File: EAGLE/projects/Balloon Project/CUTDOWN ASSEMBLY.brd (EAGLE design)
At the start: 100 x 100 mm, 2 parts

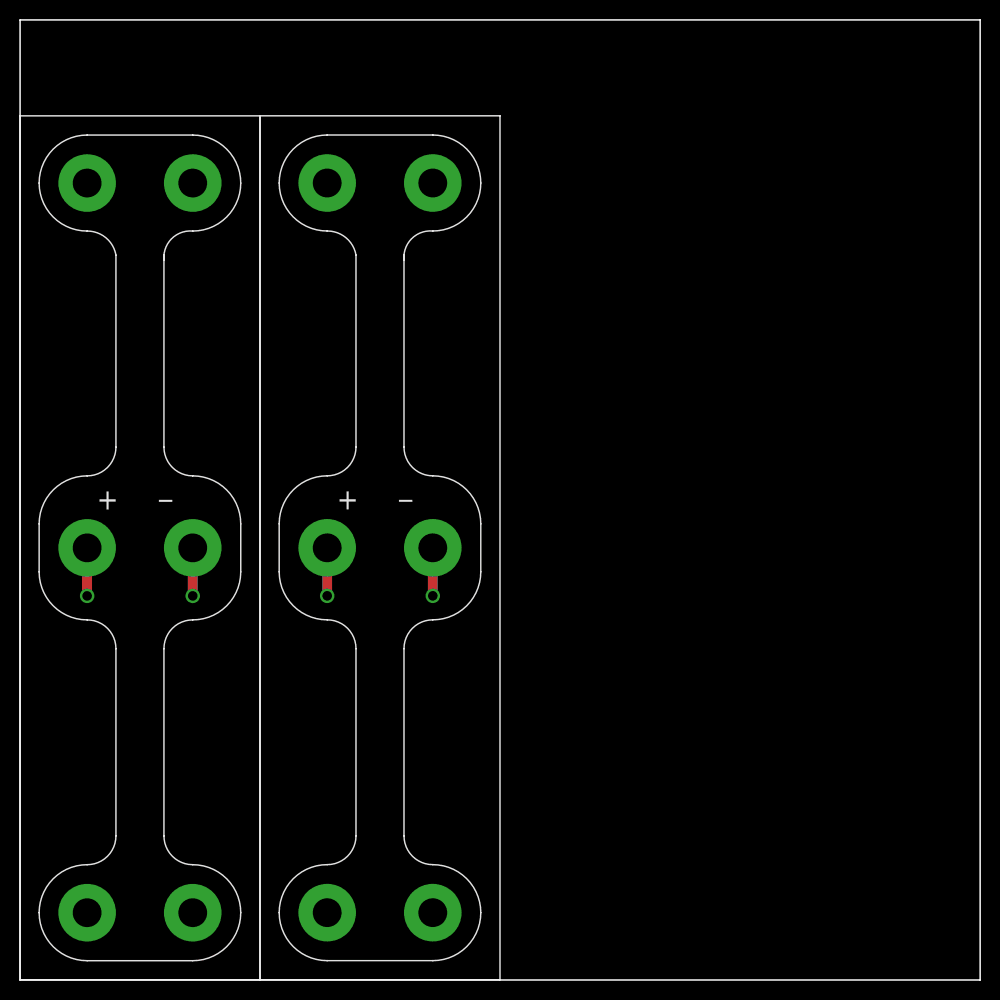
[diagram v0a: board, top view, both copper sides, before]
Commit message: gerber files generated
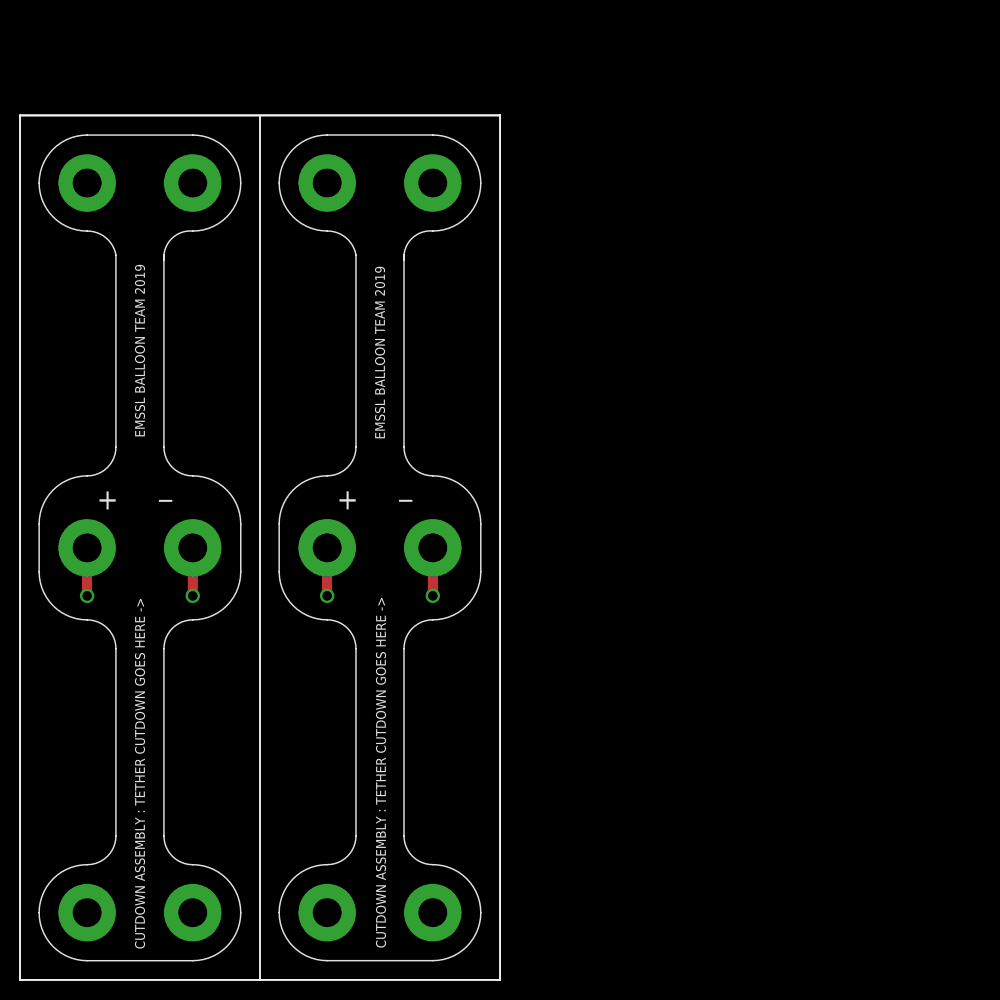
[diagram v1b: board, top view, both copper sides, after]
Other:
- board size 100 x 100 mm -> 50 x 90.1 mm
- board text added: "+"
- board text added: "CUTDOWN ASSEMBLY : TETHER CUTDOWN GOES HERE ->"
- board text added: "EMSSL BALLOON TEAM 2019"
- board text added: "_"
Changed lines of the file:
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@@
 <board>
 <plain>
-<wire x1="0" y1="0" x2="0" y2="100" width="0.1524" layer="20"/>
-<wire x1="0" y1="100" x2="100" y2="100" width="0.1524" layer="20"/>
-<wire x1="100" y1="100" x2="100" y2="0" width="0.1524" layer="20"/>
-<wire x1="100" y1="0" x2="0" y2="0" width="0.1524" layer="20"/>
+<wire x1="0" y1="0" x2="0" y2="90.1" width="0.1524" layer="20"/>
+<wire x1="0" y1="90.1" x2="50" y2="90.1" width="0.1524" layer="20"/>
+<wire x1="50" y1="90.1" x2="50" y2="0" width="0.1524" layer="20"/>
+<wire x1="50" y1="0" x2="0" y2="0" width="0.1524" layer="20"/>
+<text x="13" y="56.5" size="1.016" layer="21" rot="R90">EMSSL BALLOON TEAM 2019</text>
+<text x="38" y="56.3" size="1.016" layer="21" rot="R90">EMSSL BALLOON TEAM 2019</text>
+<text x="38.1" y="3.3" size="1.016" layer="21" rot="R90">CUTDOWN ASSEMBLY : TETHER CUTDOWN GOES HERE -&gt;</text>
+<text x="13" y="3.2" size="1.016" layer="21" rot="R90">CUTDOWN ASSEMBLY : TETHER CUTDOWN GOES HERE -&gt;</text>
+<text x="37.1" y="3.3" size="1.016" layer="22" rot="MR90">CUTDOWN ASSEMBLY : TETHER CUTDOWN GOES HERE -&gt;</text>
+<text x="12" y="3.2" size="1.016" layer="22" rot="MR90">CUTDOWN ASSEMBLY : TETHER CUTDOWN GOES HERE -&gt;</text>
+<text x="37" y="56.3" size="1.016" layer="22" rot="MR90">EMSSL BALLOON TEAM 2019</text>
+<text x="12" y="56.5" size="1.016" layer="22" rot="MR90">EMSSL BALLOON TEAM 2019</text>
+<text x="41.2" y="50.6" size="2.1844" layer="22" rot="MR0">_</text>
+<text x="16.2" y="50.6" size="2.1844" layer="22" rot="MR0">_</text>
+<text x="34.8" y="49" size="2.1844" layer="22" rot="MR0">+</text>
+<text x="9.8" y="49" size="2.1844" layer="22" rot="MR0">+</text>
 </plain>
 <attributes>
